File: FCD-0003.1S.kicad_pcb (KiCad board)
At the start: 2 copper layers, 124.2 x 75.7 mm, 22 parts, among them J1 Cartridge Edge Connector, J2 Cartridge Slot, J3 DB25_Male, J4 Jumper, J5 Jumper, J6 Jumper, U1 ATF1508AS-15JC84, U2 SST29LE010, U3 SST29LE010

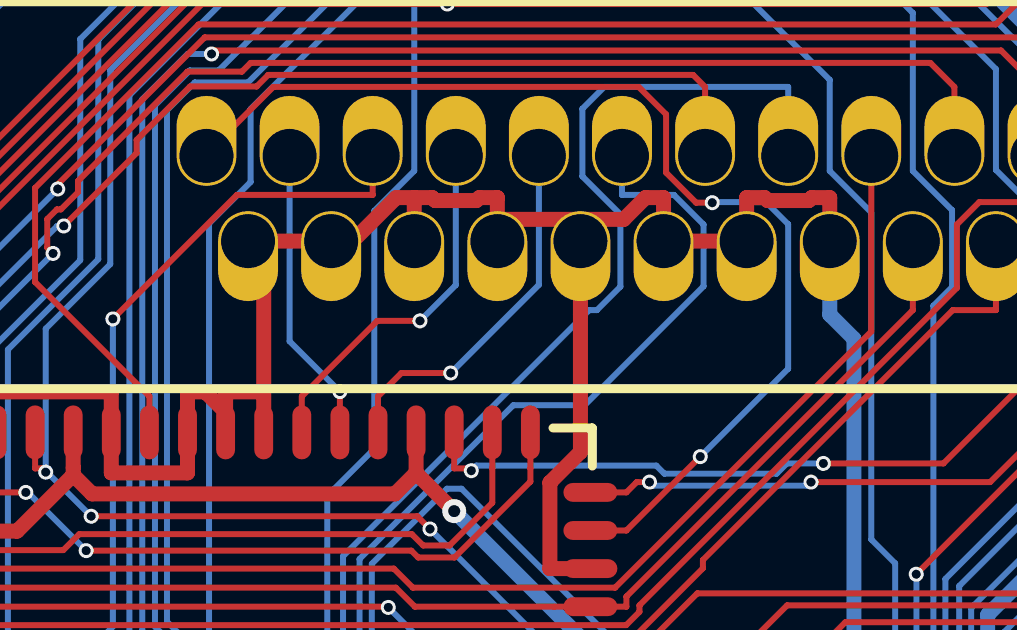
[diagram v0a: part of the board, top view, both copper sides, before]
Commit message: Add files via upload
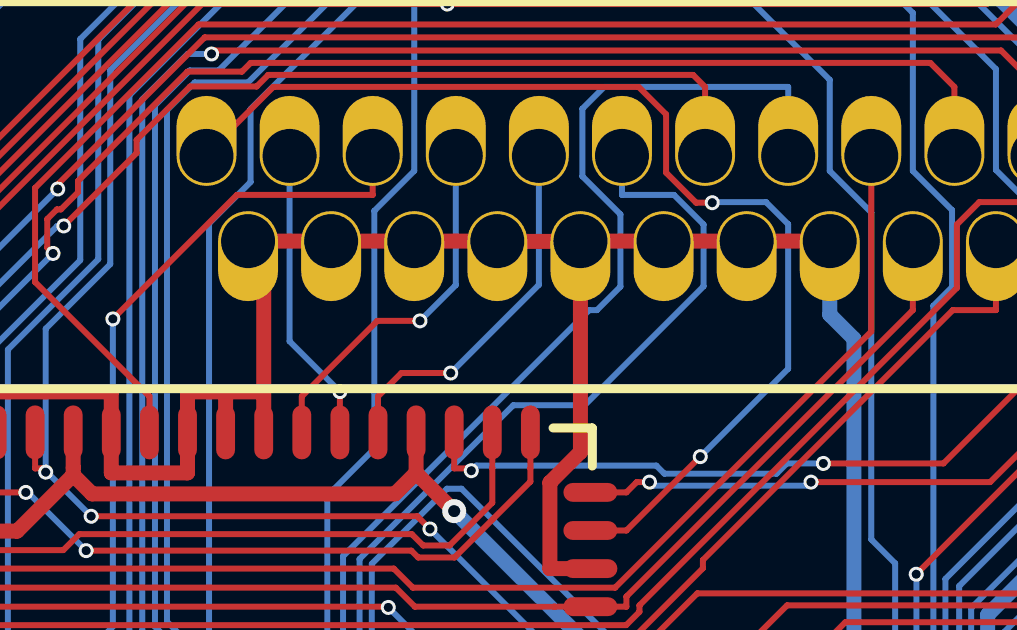
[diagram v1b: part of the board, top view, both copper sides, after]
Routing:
- net /GND: track 582.2 -> 573.9 mm
